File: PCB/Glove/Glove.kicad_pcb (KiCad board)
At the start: 2 copper layers, 70 x 70 mm, 36 parts, among them J1 JST-PH-SM4-TB, J2 USB-C-Socket-V, J3 Wago, J4 Reset, J5 BTN, J7 TC2030-USB-NL-DS, Q1 CJ2301, Q3 CJ2301, U1 ESP32-S3-MINI-1, U3 TP4054, U4 ME6211C33M5G-N

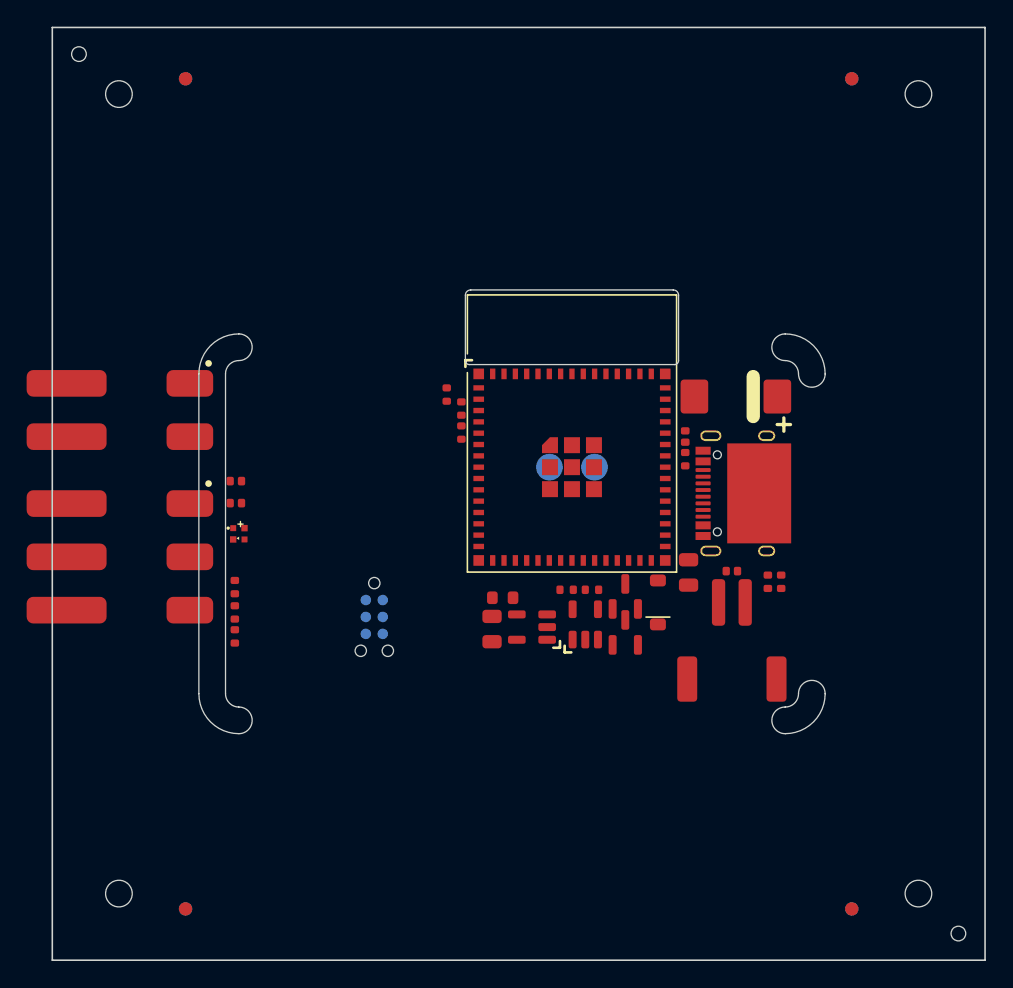
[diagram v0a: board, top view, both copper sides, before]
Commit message: Ready to track
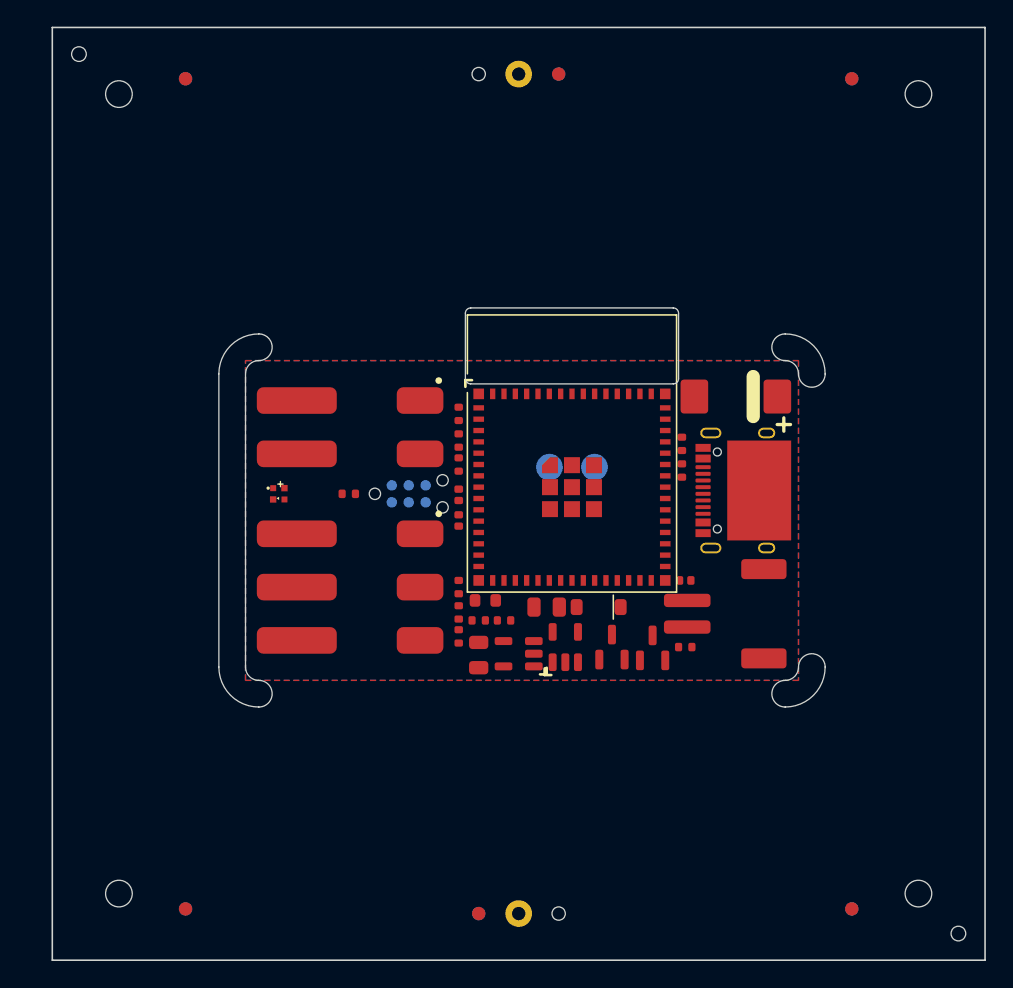
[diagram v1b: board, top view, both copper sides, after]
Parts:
- removed D24: ~, RevK:DFN1006-2L
- added R6: 10K, RevK:R_0402, F.Cu at (87.2, 100.0)
- moved J3 17.4 mm to (88.0, 107.0)
- moved J5 17.3 mm to (88.0, 95.0)
- moved D1 17.0 mm to (95.5, 102.0), turned to 90 degrees
- moved R7 16.8 mm to (95.5, 108.9)
- moved R8 16.8 mm to (95.5, 110.7)
- moved R9 16.8 mm to (95.5, 107.0)
- moved D3 16.7 mm to (95.5, 100.1), turned to 90 degrees
- moved R11 14.1 mm to (112.5, 111.5), turned to 0 degrees
- moved R3 12.8 mm to (112.2, 96.2)
- moved C26 11.0 mm to (102.0, 108.5), turned to 180 degrees
- moved R2 10.6 mm to (112.2, 98.2), turned to 90 degrees
- moved J7 9.59 mm to (91.8, 100.0), turned to 0 degrees
- moved R4 6.99 mm to (97.0, 109.5)
- moved R5 6.99 mm to (98.9, 109.5)
- moved D2 4.46 mm to (106.0, 108.5), turned to 180 degrees
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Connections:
- J3 pad 3: VBAT -> +3.3V
- U1 pad 23: unconnected-(U1-GPIO19-Pad23) -> D-
- U1 pad 4: Net-(U1-GPIO0) -> unconnected-(U1-GPIO0-Pad4)
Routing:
- added copper zone on B.Cu, net GND
- added copper zone on F.Cu, net GND
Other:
- board text added: "ironman.revk.uk"
- board text removed: "+"
- board text removed: "2 3 4 5 6 7 8 9 10 11 12 13 14 15"
- board text removed: "5060634238182"
- board text removed: "<"
- board text removed: ">"
- board text removed: "AB"
- board text removed: "C"
- board text removed: "RGB GPSTICK CHARGING GPSRX USB GPSTX SDSS SDMOSI SDSCK SDCD SDMISO ACCSDA ACCSCL PWR"
- board text removed: "S"
- board text removed: "gps.revk.uk"
- board text removed: "⎍"
- board text removed: "⏚"
